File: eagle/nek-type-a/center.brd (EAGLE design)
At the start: 55 x 70 mm, 8 parts, among them IC1 MCP23017SP

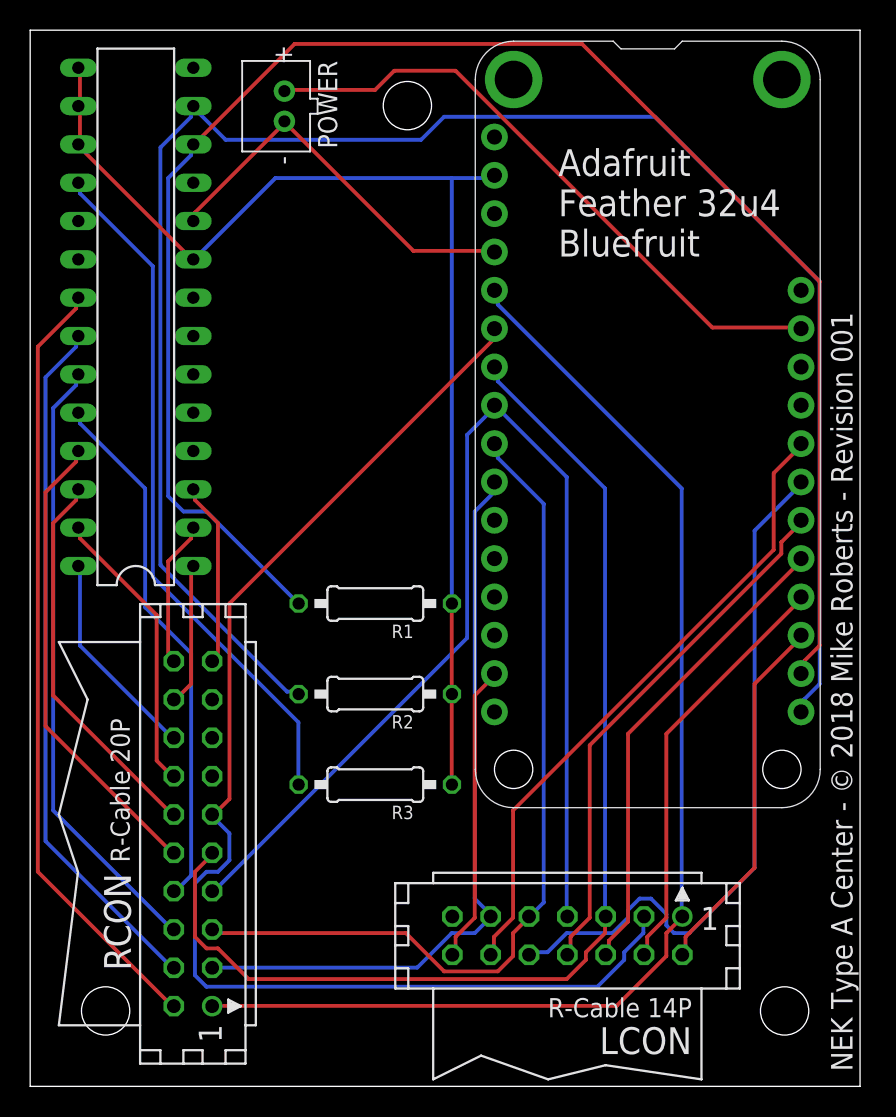
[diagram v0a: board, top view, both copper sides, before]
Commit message: logo
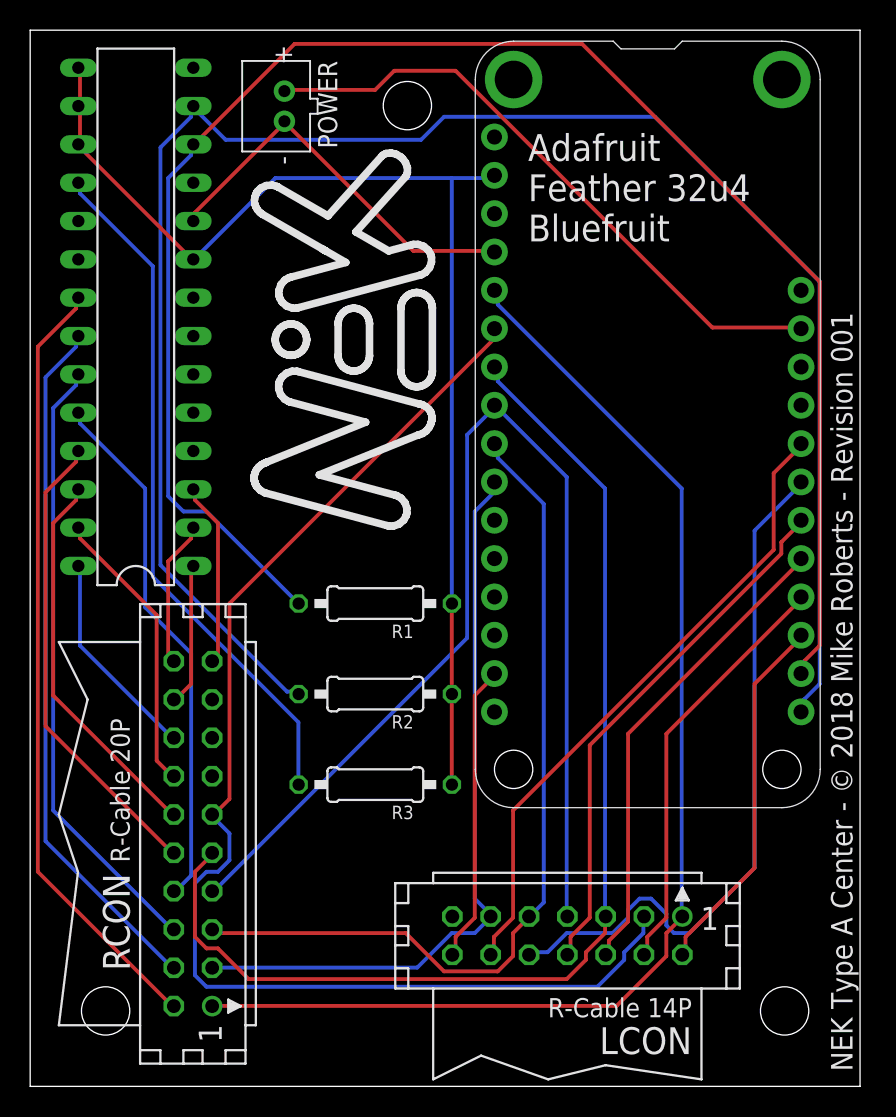
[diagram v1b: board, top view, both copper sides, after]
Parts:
- IC1: value MCP23017SP -> MCP23017E-S/P
